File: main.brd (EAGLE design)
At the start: 23.6 x 22.9 mm, 18 parts, among them U1 433MHz, U2 ATMEGA328P-MU-QFN32

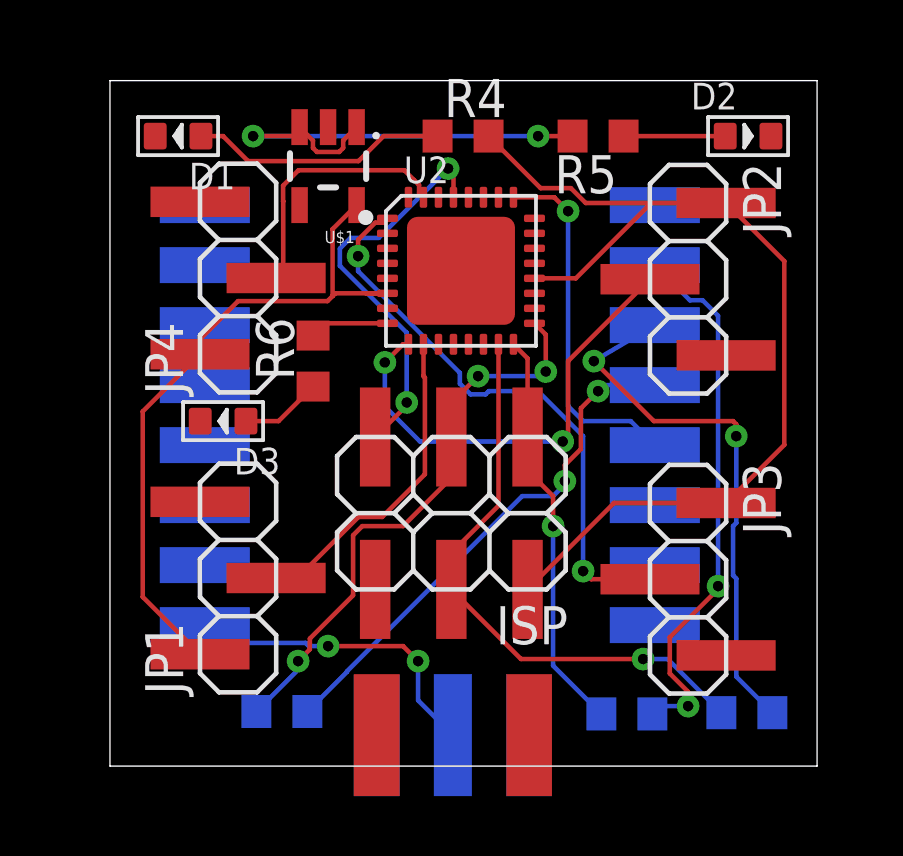
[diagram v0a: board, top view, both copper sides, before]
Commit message: Redesign
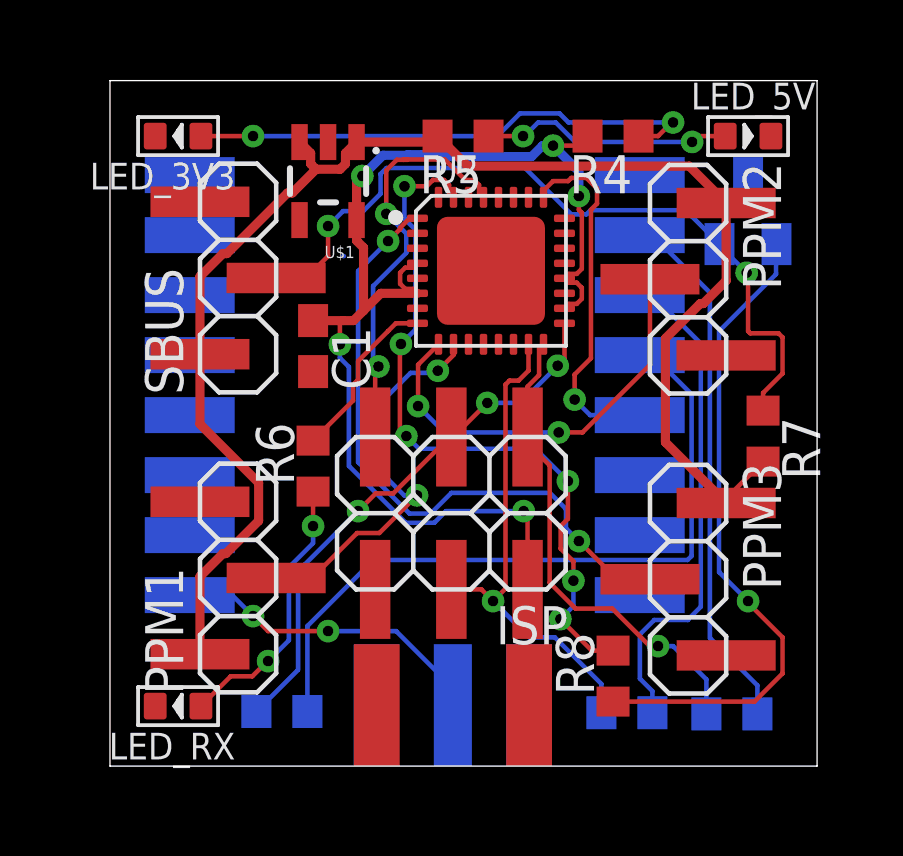
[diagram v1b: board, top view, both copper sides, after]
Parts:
- removed D3: BLUE-0603, Seeed-LED:LED-0603
- added C1: 2.2µ, resistor:C0603
- added LED_RX: BLUE-0603, Seeed-LED:LED-0603
- added Q1: BSS84, transistor-small-signal:SOT23
- added R7, R8: (no value), resistor:R0603
- moved R4 5.00 mm to (15.5, 22.0), turned to 180 degrees
- moved R5 4.50 mm to (10.5, 22.0)
- moved R2 4.00 mm to (16.0, 2.78)
- moved R3 3.50 mm to (19.5, 2.74)
- moved R6 3.50 mm to (5.50, 11.0)
- moved U1 1.12 mm to (8.89, 13.7)
- moved U2 1.00 mm to (11.4, 17.5)
- moved X1 1.00 mm to (10.2, 1.00)
- moved U$1 0.50 mm to (6.00, 20.5)
- renumbered D1 to LED_3V3, D2 to LED_5V, JP1 to PPM1, JP2 to PPM2, JP3 to PPM3, JP4 to SBUS
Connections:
- removed net PPM4: SBUS.2, U2.31
- new net !SBUS: R8.2, U2.31
- new net N$10: Q1.1, R8.1
- new net SBUS: Q1.2, R7.1, SBUS.2
- net +3V3: now also C1.1; no longer PPM1.1, PPM2.1, PPM3.1, SBUS.1
- net +5V: now also PPM1.1, PPM2.1, PPM3.1, R7.2, SBUS.1
- net GND: now also C1.2, LED_RX.-, Q1.3, U2.33; no longer D3.-
- net N$5: now also LED_RX.+; no longer D3.+
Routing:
- net +5V: track 15.3 -> 49.6 mm, vias 2 -> 0
- net SBUS: track 0.00 -> 25.7 mm, vias 0 -> 2
- net !SBUS: track 0.00 -> 24.2 mm, vias 0 -> 6
- net N$10: track 0.00 -> 22.0 mm, vias 0 -> 1
- net +3V3: track 56.2 -> 39.9 mm, vias 0 -> 5
- net N$7: track 8.58 -> 17.5 mm, vias 0 -> 2
- net PPM4: track 8.60 -> 0.00 mm
- net N$2: track 17.3 -> 24.3 mm, vias 2 -> 0
- net N$5: track 2.71 -> 9.13 mm, vias 0 -> 2
- net N$8: track 3.39 -> 8.42 mm, vias 0 -> 2
- net STATUS: track 2.65 -> 5.77 mm
- net MOSI: track 19.5 -> 16.5 mm
- net PPM1: track 10.7 -> 13.5 mm, vias 0 -> 2
- net MISO: track 13.7 -> 16.2 mm
- net PPM3: track 19.2 -> 21.4 mm
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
